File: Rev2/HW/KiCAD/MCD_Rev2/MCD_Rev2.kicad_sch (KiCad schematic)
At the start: 75 parts, among them J1 DBUS_LOW, J2 DBUS_HIGH, J3 ABUS, J4 POWER, J5 JTAG, J6 Conn_01x02_Male, J7 DUART A, J8 DUART B, SW1 SW_Push, U1 XC9572XL-PC44, U10 STM1001LWX6F, U2 AS6C1008-55PCN, U3 AS6C1008-55PCN, U4 SST39SF020A-70-4C-PHE, U5 SST39SF020A-70-4C-PHE, U6 XR68C681CJ-F, U7 AP2114HA-3.3TRG1, U8 MAX6816EUS_T, U9 MC68000FN, Y1 ECS-100AX-036, Y2 ECS-100AX-080

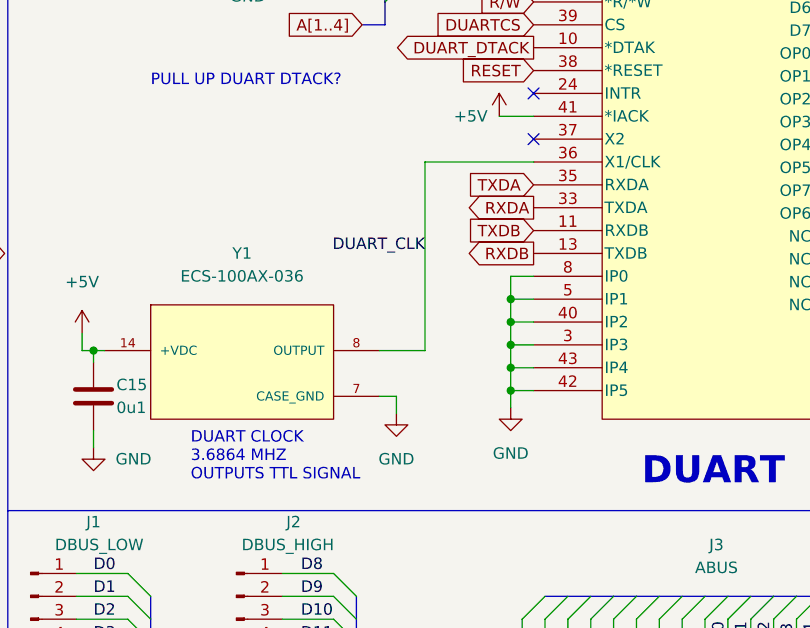
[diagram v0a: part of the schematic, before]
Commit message: finished pcb
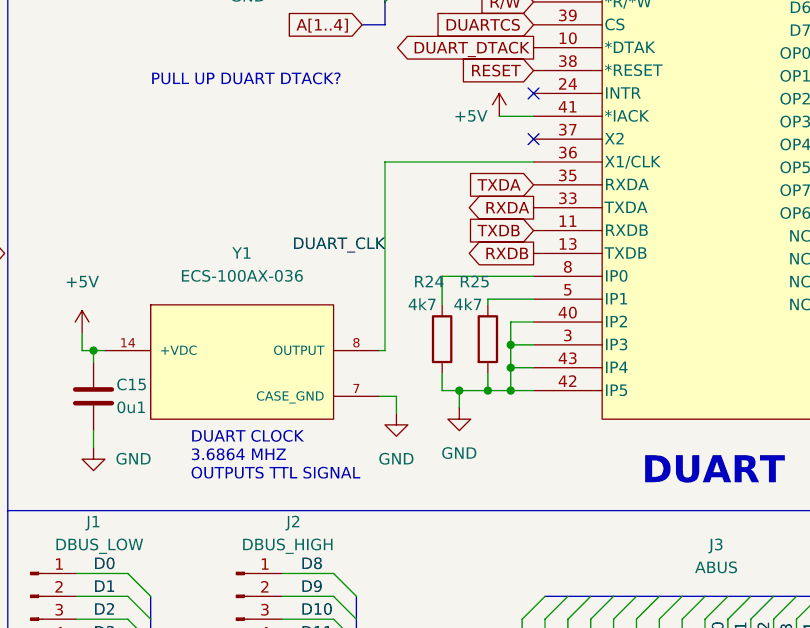
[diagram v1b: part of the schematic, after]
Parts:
- added R24, R25: 4k7, Resistor_SMD:R_0805_2012Metric_Pad1.20x1.40mm_HandSolder, symbol Device:R
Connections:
- net GND: now also R24.2, R25.2; no longer U6.5 (IP1), U6.8 (IP0)
- new net: R25.1, U6.5 (IP1)
- new net: R24.1, U6.8 (IP0)
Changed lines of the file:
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@@
   (junction (at 140.97 232.41) (diameter 0) (color 0 0 0 0)
   )
-  (junction (at 216.535 213.36) (diameter 0) (color 0 0 0 0)
-  )
   (junction (at 216.535 218.44) (diameter 0) (color 0 0 0 0)
   )
@@
   (junction (at 93.98 163.83) (diameter 0) (color 0 0 0 0)
   )
+  (junction (at 213.995 223.52) (diameter 0) (color 0 0 0 0)
+  )
   (junction (at 26.67 97.79) (diameter 0) (color 0 0 0 0)
   )
@@
   (junction (at 101.6 185.42) (diameter 0) (color 0 0 0 0)
   )
-  (junction (at 216.535 215.9) (diameter 0) (color 0 0 0 0)
-  )
   (junction (at 242.57 86.995) (diameter 0) (color 0 0 0 0)
   )
   (junction (at 26.67 36.83) (diameter 0) (color 0 0 0 0)
   )
+  (junction (at 210.82 223.52) (diameter 0) (color 0 0 0 0)
+  )
   (junction (at 129.54 232.41) (diameter 0) (color 0 0 0 0)
   )
@@
     (stroke (width 0) (type default) (color 0 0 0 0))
   )
-  (wire (pts (xy 207.01 198.12) (xy 207.01 219.075))
+  (wire (pts (xy 202.565 198.12) (xy 202.565 219.075))
     (stroke (width 0) (type default) (color 0 0 0 0))
   )
@@
     (stroke (width 0) (type default) (color 0 0 0 0))
   )
-  (wire (pts (xy 219.075 198.12) (xy 207.01 198.12))
+  (wire (pts (xy 219.075 198.12) (xy 202.565 198.12))
     (stroke (width 0) (type default) (color 0 0 0 0))
   )
@@
     (stroke (width 0) (type default) (color 0 0 0 0))
   )
+  (wire (pts (xy 208.915 223.52) (xy 210.82 223.52))
+    (stroke (width 0) (type default) (color 0 0 0 0))
+  )
   (wire (pts (xy 304.8 189.865) (xy 304.8 192.405))
     (stroke (width 0) (type default) (color 0 0 0 0))
@@
     (stroke (width 0) (type default) (color 0 0 0 0))
   )
-  (wire (pts (xy 216.535 215.9) (xy 216.535 213.36))
-    (stroke (width 0) (type default) (color 0 0 0 0))
-  )
   (bus (pts (xy 398.145 118.11) (xy 398.145 120.65))
     (stroke (width 0) (type default) (color 0 0 0 0))
@@
     (stroke (width 0) (type default) (color 0 0 0 0))
   )
+  (wire (pts (xy 210.82 223.52) (xy 210.82 225.425))
+    (stroke (width 0) (type default) (color 0 0 0 0))
+  )
   (wire (pts (xy 168.275 256.54) (xy 173.99 256.54))
     (stroke (width 0) (type default) (color 0 0 0 0))
@@
     (stroke (width 0) (type default) (color 0 0 0 0))
   )
-  (wire (pts (xy 216.535 225.425) (xy 216.535 223.52))
-    (stroke (width 0) (type default) (color 0 0 0 0))
-  )
   (wire (pts (xy 302.26 175.895) (xy 302.26 192.405))
     (stroke (width 0) (type default) (color 0 0 0 0))
@@
     (stroke (width 0) (type default) (color 0 0 0 0))
   )
+  (wire (pts (xy 213.995 213.36) (xy 213.995 213.995))
+    (stroke (width 0) (type default) (color 0 0 0 0))
+  )
   (wire (pts (xy 240.665 86.995) (xy 242.57 86.995))
     (stroke (width 0) (type default) (color 0 0 0 0))
@@
     (stroke (width 0) (type default) (color 0 0 0 0))
   )
-  (wire (pts (xy 207.01 219.075) (xy 201.93 219.075))
+  (wire (pts (xy 202.565 219.075) (xy 201.93 219.075))
     (stroke (width 0) (type default) (color 0 0 0 0))
   )
@@
     (stroke (width 0) (type default) (color 0 0 0 0))
   )
+  (wire (pts (xy 219.075 210.82) (xy 208.915 210.82))
+    (stroke (width 0) (type default) (color 0 0 0 0))
+  )
   (wire (pts (xy 389.89 186.69) (xy 395.605 186.69))
     (stroke (width 0) (type default) (color 0 0 0 0))
@@
     (stroke (width 0) (type default) (color 0 0 0 0))
   )
-  (wire (pts (xy 79.375 210.82) (xy 139.7 210.82))
+  (wire (pts (xy 213.995 223.52) (xy 216.535 223.52))
     (stroke (width 0) (type default) (color 0 0 0 0))
   )
-  (wire (pts (xy 311.15 48.895) (xy 311.15 50.8))
+  (wire (pts (xy 79.375 210.82) (xy 139.7 210.82))
     (stroke (width 0) (type default) (color 0 0 0 0))
   )
-  (wire (pts (xy 216.535 210.82) (xy 216.535 213.36))
+  (wire (pts (xy 311.15 48.895) (xy 311.15 50.8))
     (stroke (width 0) (type default) (color 0 0 0 0))
   )
@@
     (stroke (width 0) (type default) (color 0 0 0 0))
   )
+  (wire (pts (xy 219.075 213.36) (xy 213.995 213.36))
+    (stroke (width 0) (type default) (color 0 0 0 0))
+  )
   (wire (pts (xy 242.57 86.995) (xy 242.57 88.265))
     (stroke (width 0) (type default) (color 0 0 0 0))
@@
     (stroke (width 0) (type default) (color 0 0 0 0))
   )
-  (wire (pts (xy 216.535 213.36) (xy 219.075 213.36))
-    (stroke (width 0) (type default) (color 0 0 0 0))
-  )
   (wire (pts (xy 260.985 254.635) (xy 260.985 248.92))
     (stroke (width 0) (type default) (color 0 0 0 0))
@@
     (stroke (width 0) (type default) (color 0 0 0 0))
   )
+  (wire (pts (xy 213.995 221.615) (xy 213.995 223.52))
+    (stroke (width 0) (type default) (color 0 0 0 0))
+  )
   (bus (pts (xy 267.335 186.055) (xy 267.335 188.595))
     (stroke (width 0) (type default) (color 0 0 0 0))
@@
     (stroke (width 0) (type default) (color 0 0 0 0))
   )
+  (wire (pts (xy 208.915 221.615) (xy 208.915 223.52))
+    (stroke (width 0) (type default) (color 0 0 0 0))
+  )
   (bus (pts (xy 398.145 135.89) (xy 398.145 138.43))
     (stroke (width 0) (type default) (color 0 0 0 0))
@@
     (stroke (width 0) (type default) (color 0 0 0 0))
   )
-  (wire (pts (xy 219.075 210.82) (xy 216.535 210.82))
-    (stroke (width 0) (type default) (color 0 0 0 0))
-  )
   (wire (pts (xy 247.015 137.795) (xy 256.54 137.795))
     (stroke (width 0) (type default) (color 0 0 0 0))
@@
     (stroke (width 0) (type default) (color 0 0 0 0))
   )
+  (wire (pts (xy 210.82 223.52) (xy 213.995 223.52))
+    (stroke (width 0) (type default) (color 0 0 0 0))
+  )
   (wire (pts (xy 213.995 102.87) (xy 218.44 102.87))
     (stroke (width 0) (type default) (color 0 0 0 0))
@@
     (stroke (width 0) (type default) (color 0 0 0 0))
   )
+  (wire (pts (xy 208.915 210.82) (xy 208.915 213.995))
+    (stroke (width 0) (type default) (color 0 0 0 0))
+  )
   (wire (pts (xy 147.32 222.885) (xy 147.32 224.79))
     (stroke (width 0) (type default) (color 0 0 0 0))
@@
     (effects (font (size 1.27 1.27)) (justify left bottom))
   )
-  (label "DUART_CLK" (at 207.01 208.28 180)
+  (label "DUART_CLK" (at 202.565 208.28 180)
     (effects (font (size 1.27 1.27)) (justify right bottom))
   )
@@
     (pin "2")
   )
-  (symbol (lib_id "power:GND") (at 216.535 225.425 0) (mirror y) (unit 1)
+  (symbol (lib_id "power:GND") (at 210.82 225.425 0) (mirror y) (unit 1)
     (in_bom yes) (on_board yes) (fields_autoplaced)
-    (property "Reference" "#PWR0106" (id 0) (at 216.535 231.775 0)
+    (property "Reference" "#PWR0106" (id 0) (at 210.82 231.775 0)
       (effects (font (size 1.27 1.27)) hide)
     )
-    (property "Value" "GND" (id 1) (at 216.535 230.505 0))
-    (property "Footprint" "" (id 2) (at 216.535 225.425 0)
+    (property "Value" "GND" (id 1) (at 210.82 230.505 0))
+    (property "Footprint" "" (id 2) (at 210.82 225.425 0)
       (effects (font (size 1.27 1.27)) hide)
     )
-    (property "Datasheet" "" (id 3) (at 216.535 225.425 0)
+    (property "Datasheet" "" (id 3) (at 210.82 225.425 0)
       (effects (font (size 1.27 1.27)) hide)
     )
@@
     (pin "1")
   )
+  (symbol (lib_id "Device:R") (at 213.995 217.805 0) (unit 1)
+    (in_bom yes) (on_board yes)
+    (property "Reference" "R25" (id 0) (at 210.82 211.4549 0)
+      (effects (font (size 1.27 1.27)) (justify left))
+    )
+    (property "Value" "4k7" (id 1) (at 210.185 213.995 0)
+      (effects (font (size 1.27 1.27)) (justify left))
+    )
+    (property "Footprint" "Resistor_SMD:R_0805_2012Metric_Pad1.20x1.40mm_HandSolder" (id 2) (at 212.217 217.805 90)
+      (effects (font (size 1.27 1.27)) hide)
+    )
+    (property "Datasheet" "~" (id 3) (at 213.995 217.805 0)
+      (effects (font (size 1.27 1.27)) hide)
+    )
+    (pin "1")
+    (pin "2")
+  )
   (symbol (lib_id "Device:R") (at 93.98 172.72 0) (unit 1)
     (in_bom yes) (on_board yes)
@@
     (pin "1")
   )
+  (symbol (lib_id "Device:R") (at 208.915 217.805 0) (unit 1)
+    (in_bom yes) (on_board yes)
+    (property "Reference" "R24" (id 0) (at 205.74 211.4549 0)
+      (effects (font (size 1.27 1.27)) (justify left))
+    )
+    (property "Value" "4k7" (id 1) (at 205.105 213.995 0)
+      (effects (font (size 1.27 1.27)) (justify left))
+    )
+    (property "Footprint" "Resistor_SMD:R_0805_2012Metric_Pad1.20x1.40mm_HandSolder" (id 2) (at 207.137 217.805 90)
+      (effects (font (size 1.27 1.27)) hide)
+    )
+    (property "Datasheet" "~" (id 3) (at 208.915 217.805 0)
+      (effects (font (size 1.27 1.27)) hide)
+    )
+    (pin "1")
+    (pin "2")
+  )
   (symbol (lib_id "Connector:Conn_01x08_Male") (at 163.195 251.46 0) (unit 1)
     (in_bom yes) (on_board yes)
@@
       (reference "R23") (unit 1) (value "1k") (footprint "Resistor_SMD:R_0805_2012Metric_Pad1.20x1.40mm_HandSolder")
     )
+    (path "/f8ffca83-a86c-4a58-948c-2ec25998a0e9"
+      (reference "R24") (unit 1) (value "4k7") (footprint "Resistor_SMD:R_0805_2012Metric_Pad1.20x1.40mm_HandSolder")
+    )
+    (path "/8e3ebaeb-46e3-4d82-9340-c7f330c37873"
+      (reference "R25") (unit 1) (value "4k7") (footprint "Resistor_SMD:R_0805_2012Metric_Pad1.20x1.40mm_HandSolder")
+    )
     (path "/0462ae0a-38ba-4d29-9f39-4802b7ef4750"
